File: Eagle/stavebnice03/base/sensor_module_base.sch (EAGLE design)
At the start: 5 parts

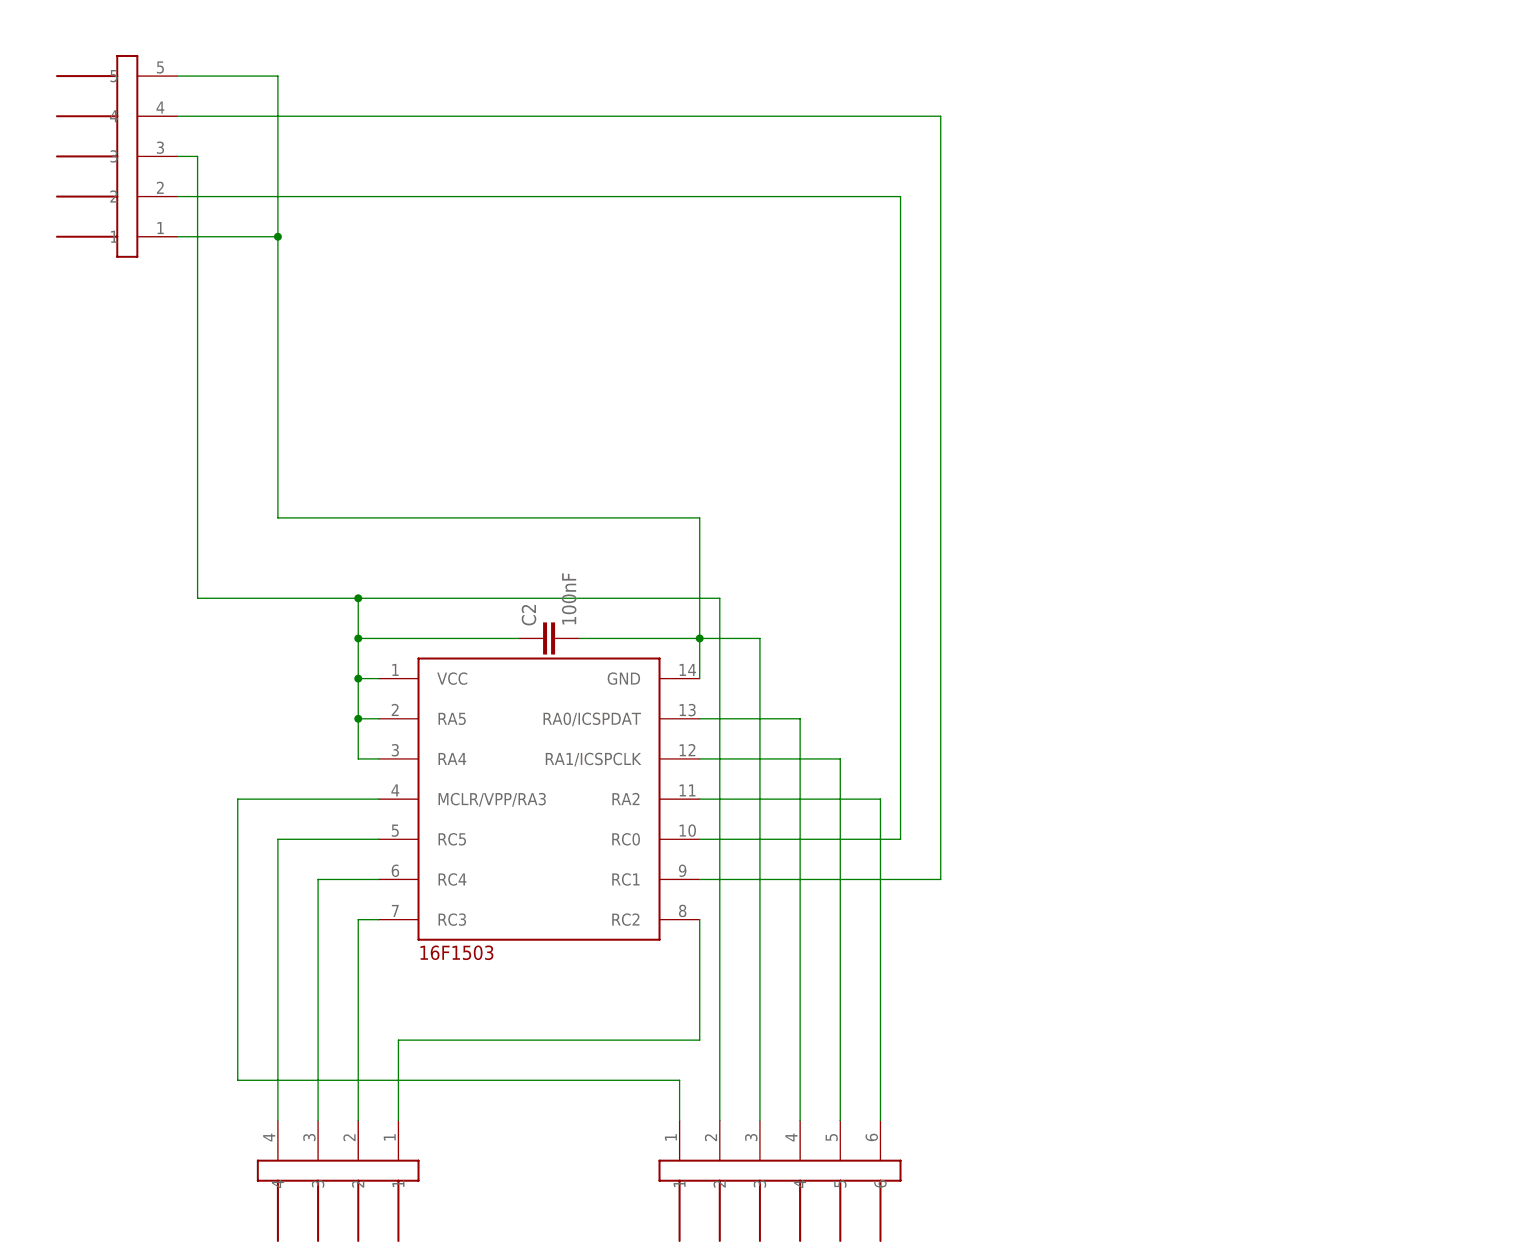
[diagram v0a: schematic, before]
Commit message: I did an order in Eagle files
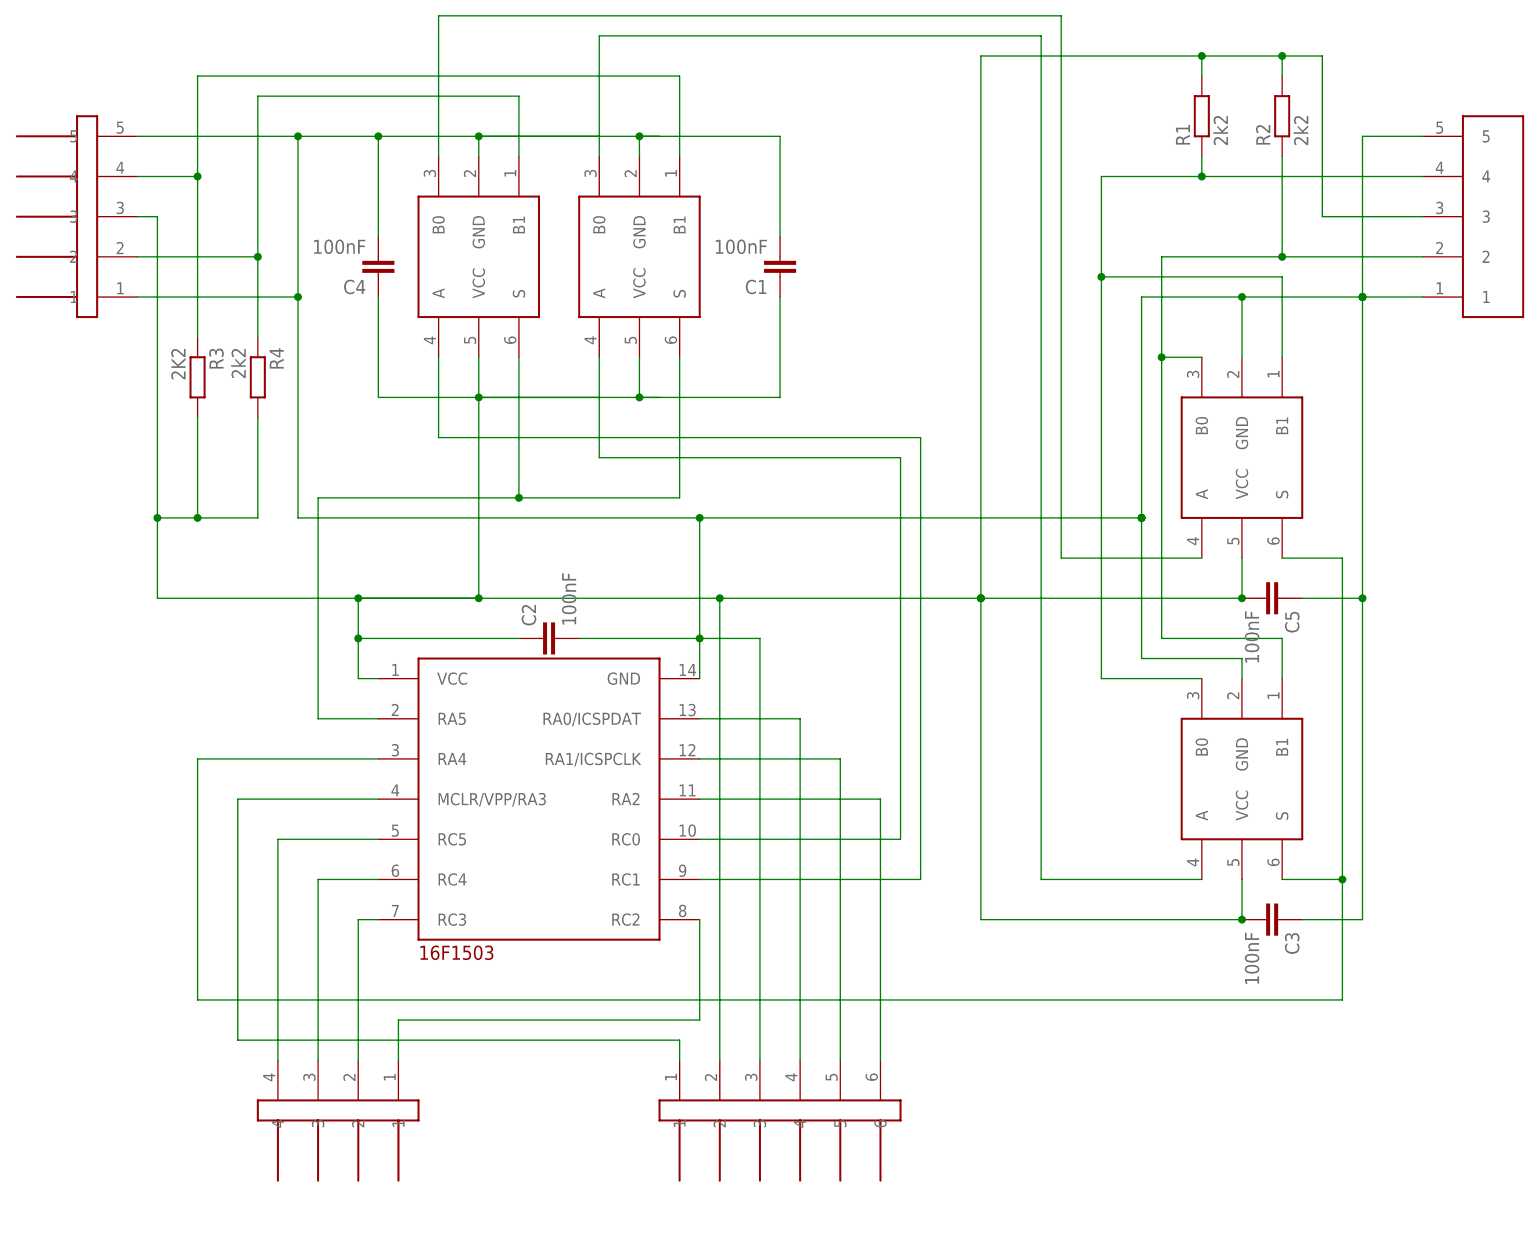
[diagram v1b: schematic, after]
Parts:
- added C1, C3, C4, C5: 100nF, resistor:C-EUC0603
- added R1, R2, R4: 2k2, resistor:R-EU_R0603
- added R3: 2K2, resistor:R-EU_R0603
- added U$2, U$3, U$6, U$7: NC7SB3157P6X, !stavebnice03:NC7SB3157P6X
- added U$5: JUMPER5F-90, !stavebnice03:JUMPER5F-90
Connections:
- new net N$1: U$1.RA4, U$6.S, U$7.S
- new net N$10: R2.1, U$5.2, U$6.B0, U$7.B1
- new net N$20: U$2.B0, U$7.A
- new net N$4: U$1.RC1, U$3.A
- new net N$6: R1.1, U$5.4, U$6.B1, U$7.B0
- new net N$7: U$3.B0, U$6.A
- new net N$8: R4.1, U$3.B1, U$4.2
- new net N$9: U$1.RA5, U$2.S, U$3.S
- net GND: now also C1.2, C3.1, C4.2, C5.1, U$2.GND, U$3.GND, U$5.1, U$5.5, U$6.GND, U$7.GND
- net N$2: now also U$2.A; no longer U$4.2
- net N$5: now also R3.1, U$2.B1; no longer U$1.RC1
- net VCC: now also C1.1, C3.2, C4.1, C5.2, R1.2, R2.2, R3.2, R4.2, U$2.VCC, U$3.VCC, U$5.3, U$6.VCC, U$7.VCC; no longer U$1.RA4, U$1.RA5
